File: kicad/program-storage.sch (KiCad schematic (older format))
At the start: 1 part

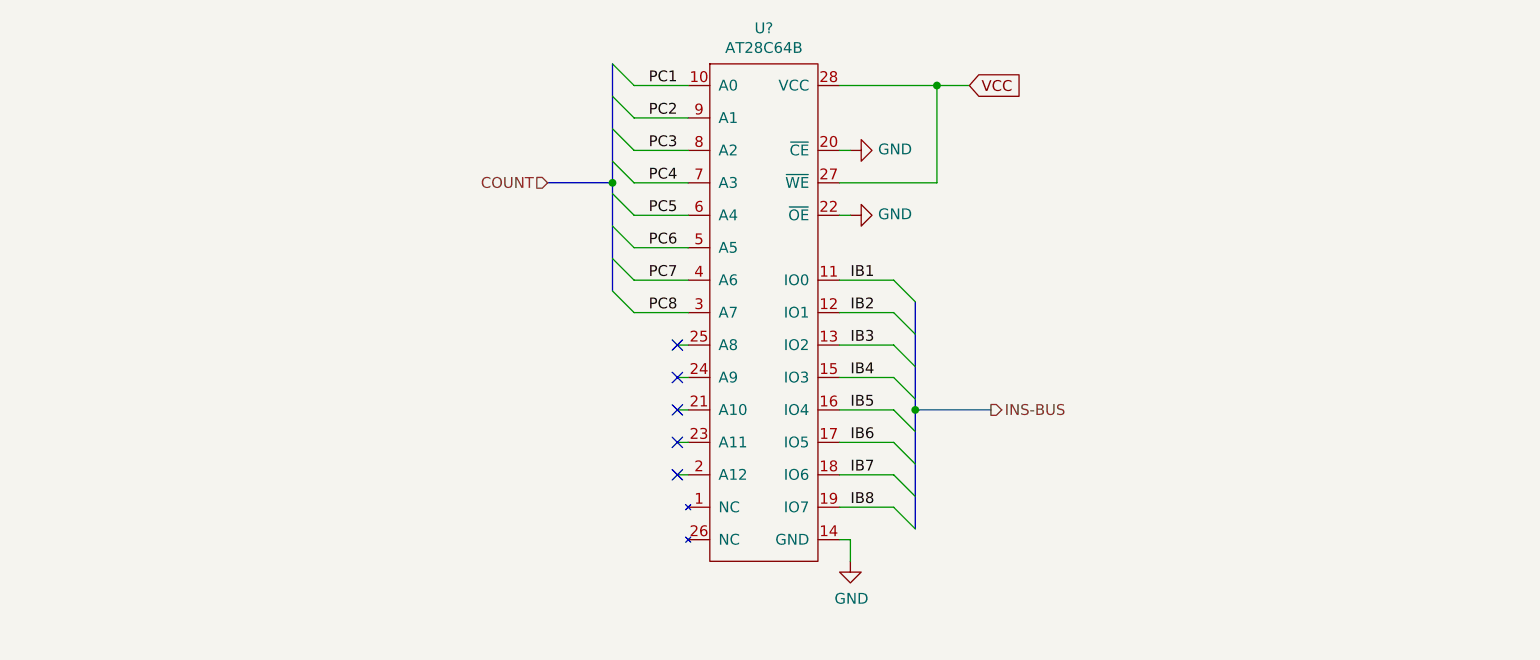
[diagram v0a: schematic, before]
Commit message: Final Commit Pre-Talk The final commit before Monday's talk, including the PDF of the schematic to make it accessible.
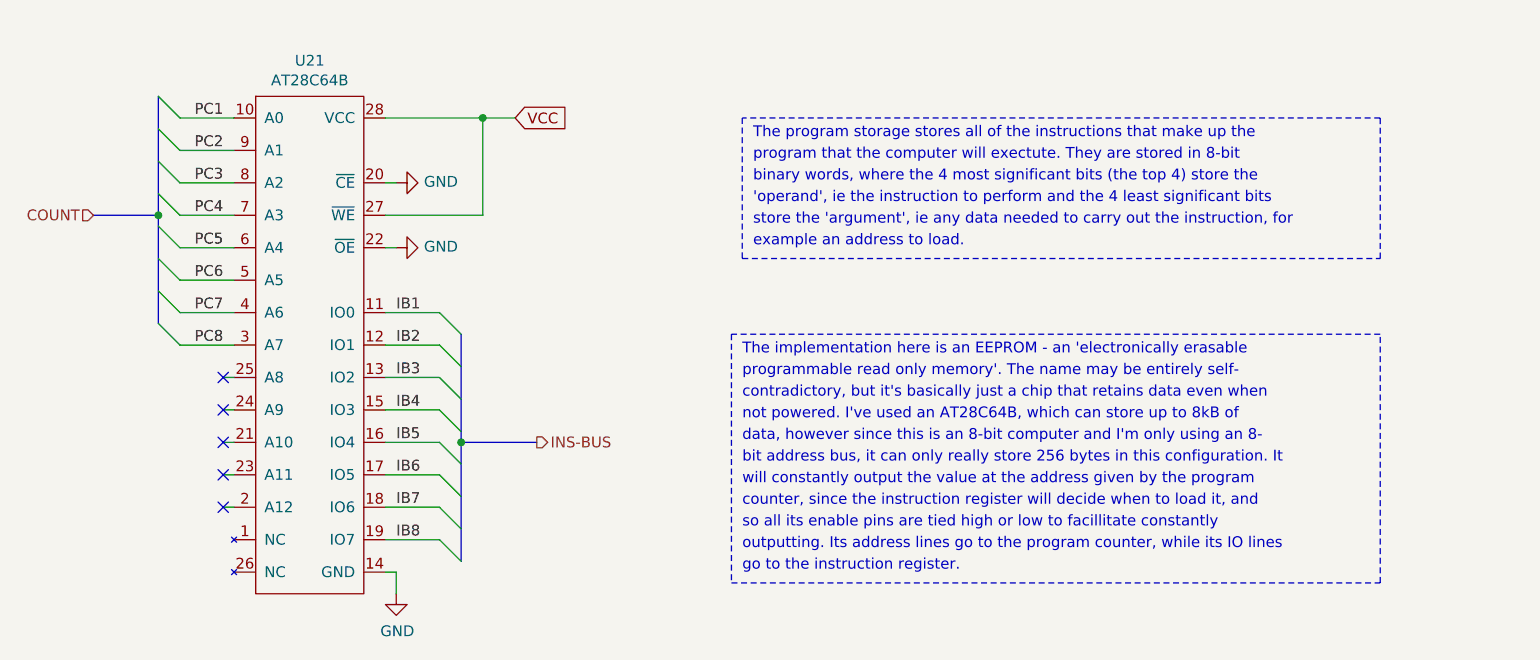
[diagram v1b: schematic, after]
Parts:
- gave numbers to parts that had none: 1
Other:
- note added: "'operand', ie the instruction to perform and the 4 least significant bits"
- note added: "The implementation here is an EEPROM - an 'electronically erasable"
- note added: "The program storage stores all of the instructions that make up the"
- note added: "binary words, where the 4 most significant bits (the top 4) store the"
- note added: "bit address bus, it can only really store 256 bytes in this configuration. It"
- note added: "contradictory, but it's basically just a chip that retains data even when"
- note added: "counter, since the instruction register will decide when to load it, and"
- note added: "data, however since this is an 8-bit computer and I'm only using an 8-"
- note added: "example an address to load."
- note added: "go to the instruction register."
- note added: "not powered. I've used an AT28C64B, which can store up to 8kB of"
- note added: "outputting. Its address lines go to the program counter, while its IO lines"
- note added: "program that the computer will exectute. They are stored in 8-bit"
- note added: "programmable read only memory'. The name may be entirely self-"
- note added: "so all its enable pins are tied high or low to facillitate constantly"
- note added: "store the 'argument', ie any data needed to carry out the instruction, for"
- note added: "will constantly output the value at the address given by the program"
- moved on the sheet: U21
